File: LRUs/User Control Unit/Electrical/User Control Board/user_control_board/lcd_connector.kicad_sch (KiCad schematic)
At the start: 1 part

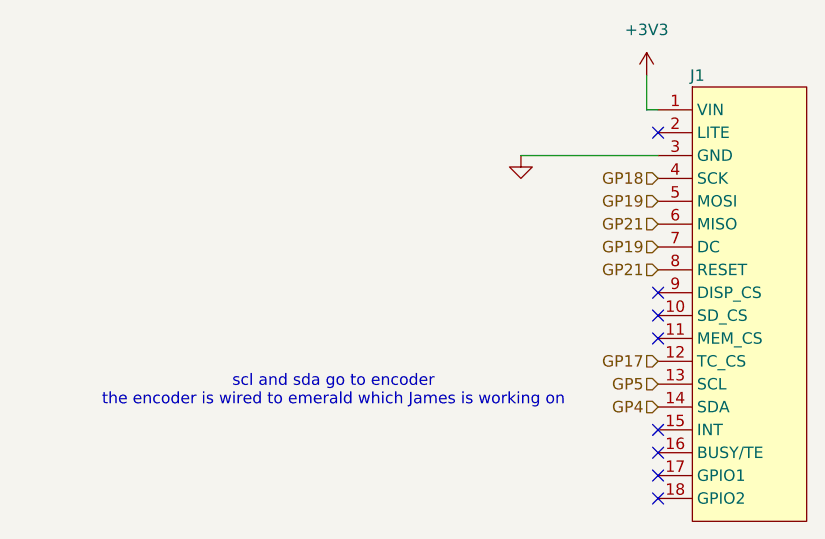
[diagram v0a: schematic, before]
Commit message: need to run DCR
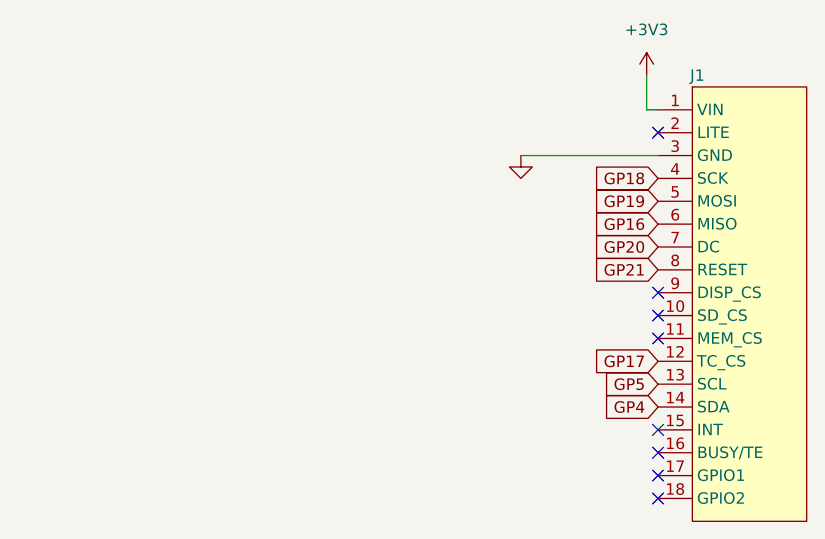
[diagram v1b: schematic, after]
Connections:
- net GP19: no longer J1.7 (DC)
- net GP21: no longer J1.6 (MISO)
- new net GP16: J1.6 (MISO)
- new net GP20: J1.7 (DC)
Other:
- note removed: "scl and sda go to encoder the encoder is wired to emerald which James is working on"
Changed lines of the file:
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@@
 	(generator_version "10.0")
 	(paper "A4")
-	(text "scl and sda go to encoder\nthe encoder is wired to emerald which James is working on"
-		(exclude_from_sim no)
-		(at 162.052 106.172 0)
-		(effects
-			(font
-				(size 1.27 1.27)
-			)
-		)
-	)
 	(no_connect
 		(at 198.12 113.03)
@@
 		)
 	)
-	(hierarchical_label "GP21"
+	(global_label "GP20"
+		(shape input)
+		(at 198.12 90.17 180)
+		(fields_autoplaced yes)
+		(effects
+			(font
+				(size 1.27 1.27)
+			)
+			(justify right)
+		)
+		(property "Intersheetrefs" "${INTERSHEET_REFS}"
+			(at 190.1758 90.17 0)
+			(hide yes)
+			(show_name no)
+			(do_not_autoplace no)
+			(effects
+				(font
+					(size 1.27 1.27)
+				)
+				(justify right)
+			)
+		)
+	)
+	(global_label "GP5"
+		(shape input)
+		(at 198.12 105.41 180)
+		(fields_autoplaced yes)
+		(effects
+			(font
+				(size 1.27 1.27)
+			)
+			(justify right)
+		)
+		(property "Intersheetrefs" "${INTERSHEET_REFS}"
+			(at 191.3853 105.41 0)
+			(hide yes)
+			(show_name no)
+			(do_not_autoplace no)
+			(effects
+				(font
+					(size 1.27 1.27)
+				)
+				(justify right)
+			)
+		)
+	)
+	(global_label "GP18"
+		(shape input)
+		(at 198.12 82.55 180)
+		(fields_autoplaced yes)
+		(effects
+			(font
+				(size 1.27 1.27)
+			)
+			(justify right)
+		)
+		(property "Intersheetrefs" "${INTERSHEET_REFS}"
+			(at 190.1758 82.55 0)
+			(hide yes)
+			(show_name no)
+			(do_not_autoplace no)
+			(effects
+				(font
+					(size 1.27 1.27)
+				)
+				(justify right)
+			)
+		)
+	)
+	(global_label "GP21"
+		(shape input)
+		(at 198.12 92.71 180)
+		(fields_autoplaced yes)
+		(effects
+			(font
+				(size 1.27 1.27)
+			)
+			(justify right)
+		)
+		(property "Intersheetrefs" "${INTERSHEET_REFS}"
+			(at 190.1758 92.71 0)
+			(hide yes)
+			(show_name no)
+			(do_not_autoplace no)
+			(effects
+				(font
+					(size 1.27 1.27)
+				)
+				(justify right)
+			)
+		)
+	)
+	(global_label "GP4"
+		(shape input)
+		(at 198.12 107.95 180)
+		(fields_autoplaced yes)
+		(effects
+			(font
+				(size 1.27 1.27)
+			)
+			(justify right)
+		)
+		(property "Intersheetrefs" "${INTERSHEET_REFS}"
+			(at 191.3853 107.95 0)
+			(hide yes)
+			(show_name no)
+			(do_not_autoplace no)
+			(effects
+				(font
+					(size 1.27 1.27)
+				)
+				(justify right)
+			)
+		)
+	)
+	(global_label "GP17"
+		(shape input)
+		(at 198.12 102.87 180)
+		(fields_autoplaced yes)
+		(effects
+			(font
+				(size 1.27 1.27)
+			)
+			(justify right)
+		)
+		(property "Intersheetrefs" "${INTERSHEET_REFS}"
+			(at 190.1758 102.87 0)
+			(hide yes)
+			(show_name no)
+			(do_not_autoplace no)
+			(effects
+				(font
+					(size 1.27 1.27)
+				)
+				(justify right)
+			)
+		)
+	)
+	(global_label "GP16"
 		(shape input)
 		(at 198.12 87.63 180)
-		(effects
-			(font
-				(size 1.27 1.27)
-			)
-			(justify right)
-		)
-	)
-	(hierarchical_label "GP21"
-		(shape input)
-		(at 198.12 92.71 180)
-		(effects
-			(font
-				(size 1.27 1.27)
-			)
-			(justify right)
-		)
-	)
-	(hierarchical_label "GP19"
+		(fields_autoplaced yes)
+		(effects
+			(font
+				(size 1.27 1.27)
+			)
+			(justify right)
+		)
+		(property "Intersheetrefs" "${INTERSHEET_REFS}"
+			(at 190.1758 87.63 0)
+			(hide yes)
+			(show_name no)
+			(do_not_autoplace no)
+			(effects
+				(font
+					(size 1.27 1.27)
+				)
+				(justify right)
+			)
+		)
+	)
+	(global_label "GP19"
 		(shape input)
 		(at 198.12 85.09 180)
-		(effects
-			(font
-				(size 1.27 1.27)
-			)
-			(justify right)
-		)
-	)
-	(hierarchical_label "GP19"
-		(shape input)
-		(at 198.12 90.17 180)
-		(effects
-			(font
-				(size 1.27 1.27)
-			)
-			(justify right)
-		)
-	)
-	(hierarchical_label "GP5"
-		(shape input)
-		(at 198.12 105.41 180)
-		(effects
-			(font
-				(size 1.27 1.27)
-			)
-			(justify right)
-		)
-	)
-	(hierarchical_label "GP18"
-		(shape input)
-		(at 198.12 82.55 180)
-		(effects
-			(font
-				(size 1.27 1.27)
-			)
-			(justify right)
-		)
-	)
-	(hierarchical_label "GP4"
-		(shape input)
-		(at 198.12 107.95 180)
-		(effects
-			(font
-				(size 1.27 1.27)
-			)
-			(justify right)
-		)
-	)
-	(hierarchical_label "GP17"
-		(shape input)
-		(at 198.12 102.87 180)
-		(effects
-			(font
-				(size 1.27 1.27)
-			)
-			(justify right)
-		)
-	)
+		(fields_autoplaced yes)
+		(effects
+			(font
+				(size 1.27 1.27)
+			)
+			(justify right)
+		)
+		(property "Intersheetrefs" "${INTERSHEET_REFS}"
+			(at 190.1758 85.09 0)
+			(hide yes)
+			(show_name no)
+			(do_not_autoplace no)
+			(effects
+				(font
+					(size 1.27 1.27)
+				)
+				(justify right)
+			)
+		)
+	)

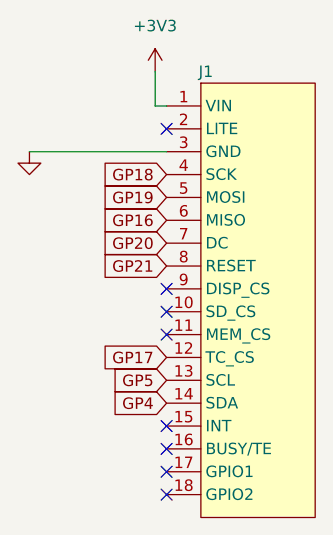
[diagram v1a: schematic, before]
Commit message: connectors and 5v buck partially done
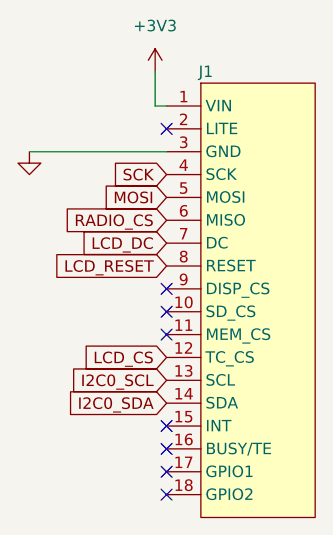
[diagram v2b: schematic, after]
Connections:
- net GP16 renamed RADIO_CS
- net GP17 renamed LCD_CS
- net GP18 renamed SCK
- net GP19 renamed MOSI
- net GP20 renamed LCD_DC
- net GP21 renamed LCD_RESET
- net GP4 renamed I2C0_SDA
- net GP5 renamed I2C0_SCL
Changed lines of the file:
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@@
 		)
 	)
-	(global_label "GP20"
+	(global_label "LCD_DC"
 		(shape input)
 		(at 198.12 90.17 180)
@@
 		)
 		(property "Intersheetrefs" "${INTERSHEET_REFS}"
-			(at 190.1758 90.17 0)
-			(hide yes)
-			(show_name no)
-			(do_not_autoplace no)
-			(effects
-				(font
-					(size 1.27 1.27)
-				)
-				(justify right)
-			)
-		)
-	)
-	(global_label "GP5"
+			(at 188.0591 90.17 0)
+			(hide yes)
+			(show_name no)
+			(do_not_autoplace no)
+			(effects
+				(font
+					(size 1.27 1.27)
+				)
+				(justify right)
+			)
+		)
+	)
+	(global_label "I2C0_SDA"
+		(shape input)
+		(at 198.12 107.95 180)
+		(fields_autoplaced yes)
+		(effects
+			(font
+				(size 1.27 1.27)
+			)
+			(justify right)
+		)
+		(property "Intersheetrefs" "${INTERSHEET_REFS}"
+			(at 186.3053 107.95 0)
+			(hide yes)
+			(show_name no)
+			(do_not_autoplace no)
+			(effects
+				(font
+					(size 1.27 1.27)
+				)
+				(justify right)
+			)
+		)
+	)
+	(global_label "SCK"
+		(shape input)
+		(at 198.12 82.55 180)
+		(fields_autoplaced yes)
+		(effects
+			(font
+				(size 1.27 1.27)
+			)
+			(justify right)
+		)
+		(property "Intersheetrefs" "${INTERSHEET_REFS}"
+			(at 191.3853 82.55 0)
+			(hide yes)
+			(show_name no)
+			(do_not_autoplace no)
+			(effects
+				(font
+					(size 1.27 1.27)
+				)
+				(justify right)
+			)
+		)
+	)
+	(global_label "LCD_RESET"
+		(shape input)
+		(at 198.12 92.71 180)
+		(fields_autoplaced yes)
+		(effects
+			(font
+				(size 1.27 1.27)
+			)
+			(justify right)
+		)
+		(property "Intersheetrefs" "${INTERSHEET_REFS}"
+			(at 184.854 92.71 0)
+			(hide yes)
+			(show_name no)
+			(do_not_autoplace no)
+			(effects
+				(font
+					(size 1.27 1.27)
+				)
+				(justify right)
+			)
+		)
+	)
+	(global_label "LCD_CS"
+		(shape input)
+		(at 198.12 102.87 180)
+		(fields_autoplaced yes)
+		(effects
+			(font
+				(size 1.27 1.27)
+			)
+			(justify right)
+		)
+		(property "Intersheetrefs" "${INTERSHEET_REFS}"
+			(at 188.1196 102.87 0)
+			(hide yes)
+			(show_name no)
+			(do_not_autoplace no)
+			(effects
+				(font
+					(size 1.27 1.27)
+				)
+				(justify right)
+			)
+		)
+	)
+	(global_label "RADIO_CS"
+		(shape input)
+		(at 198.12 87.63 180)
+		(fields_autoplaced yes)
+		(effects
+			(font
+				(size 1.27 1.27)
+			)
+			(justify right)
+		)
+		(property "Intersheetrefs" "${INTERSHEET_REFS}"
+			(at 186.1238 87.63 0)
+			(hide yes)
+			(show_name no)
+			(do_not_autoplace no)
+			(effects
+				(font
+					(size 1.27 1.27)
+				)
+				(justify right)
+			)
+		)
+	)
+	(global_label "I2C0_SCL"
 		(shape input)
 		(at 198.12 105.41 180)
@@
 		)
 		(property "Intersheetrefs" "${INTERSHEET_REFS}"
-			(at 191.3853 105.41 0)
-			(hide yes)
-			(show_name no)
-			(do_not_autoplace no)
-			(effects
-				(font
-					(size 1.27 1.27)
-				)
-				(justify right)
-			)
-		)
-	)
-	(global_label "GP18"
-		(shape input)
-		(at 198.12 82.55 180)
-		(fields_autoplaced yes)
-		(effects
-			(font
-				(size 1.27 1.27)
-			)
-			(justify right)
-		)
-		(property "Intersheetrefs" "${INTERSHEET_REFS}"
-			(at 190.1758 82.55 0)
-			(hide yes)
-			(show_name no)
-			(do_not_autoplace no)
-			(effects
-				(font
-					(size 1.27 1.27)
-				)
-				(justify right)
-			)
-		)
-	)
-	(global_label "GP21"
-		(shape input)
-		(at 198.12 92.71 180)
-		(fields_autoplaced yes)
-		(effects
-			(font
-				(size 1.27 1.27)
-			)
-			(justify right)
-		)
-		(property "Intersheetrefs" "${INTERSHEET_REFS}"
-			(at 190.1758 92.71 0)
-			(hide yes)
-			(show_name no)
-			(do_not_autoplace no)
-			(effects
-				(font
-					(size 1.27 1.27)
-				)
-				(justify right)
-			)
-		)
-	)
-	(global_label "GP4"
-		(shape input)
-		(at 198.12 107.95 180)
-		(fields_autoplaced yes)
-		(effects
-			(font
-				(size 1.27 1.27)
-			)
-			(justify right)
-		)
-		(property "Intersheetrefs" "${INTERSHEET_REFS}"
-			(at 191.3853 107.95 0)
-			(hide yes)
-			(show_name no)
-			(do_not_autoplace no)
-			(effects
-				(font
-					(size 1.27 1.27)
-				)
-				(justify right)
-			)
-		)
-	)
-	(global_label "GP17"
-		(shape input)
-		(at 198.12 102.87 180)
-		(fields_autoplaced yes)
-		(effects
-			(font
-				(size 1.27 1.27)
-			)
-			(justify right)
-		)
-		(property "Intersheetrefs" "${INTERSHEET_REFS}"
-			(at 190.1758 102.87 0)
-			(hide yes)
-			(show_name no)
-			(do_not_autoplace no)
-			(effects
-				(font
-					(size 1.27 1.27)
-				)
-				(justify right)
-			)
-		)
-	)
-	(global_label "GP16"
-		(shape input)
-		(at 198.12 87.63 180)
-		(fields_autoplaced yes)
-		(effects
-			(font
-				(size 1.27 1.27)
-			)
-			(justify right)
-		)
-		(property "Intersheetrefs" "${INTERSHEET_REFS}"
-			(at 190.1758 87.63 0)
-			(hide yes)
-			(show_name no)
-			(do_not_autoplace no)
-			(effects
-				(font
-					(size 1.27 1.27)
-				)
-				(justify right)
-			)
-		)
-	)
-	(global_label "GP19"
+			(at 186.3658 105.41 0)
+			(hide yes)
+			(show_name no)
+			(do_not_autoplace no)
+			(effects
+				(font
+					(size 1.27 1.27)
+				)
+				(justify right)
+			)
+		)
+	)
+	(global_label "MOSI"
 		(shape input)
 		(at 198.12 85.09 180)
@@
 		)
 		(property "Intersheetrefs" "${INTERSHEET_REFS}"
-			(at 190.1758 85.09 0)
+			(at 190.5386 85.09 0)
 			(hide yes)
 			(show_name no)
@@
 		(dnp no)
 		(fields_autoplaced yes)
-		(property "Reference" "#PWR017"
+		(property "Reference" "#PWR05"
 			(at 196.85 74.93 0)
 			(hide yes)
@@
 			(project "user_control_board"
 				(path "/bc27608c-d267-4607-a115-e0984dc927e7"
-					(reference "#PWR017")
+					(reference "#PWR05")
 					(unit 1)
 				)
@@
 		(dnp no)
 		(fields_autoplaced yes)
-		(property "Reference" "#PWR018"
+		(property "Reference" "#PWR04"
 			(at 182.88 86.36 0)
 			(hide yes)
@@
 			(project "user_control_board"
 				(path "/bc27608c-d267-4607-a115-e0984dc927e7"
-					(reference "#PWR018")
+					(reference "#PWR04")
 					(unit 1)
 				)
